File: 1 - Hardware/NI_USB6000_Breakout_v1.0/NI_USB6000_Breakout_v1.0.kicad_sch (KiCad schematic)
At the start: 19 parts, among them J1 NI_6000_CONN, J2 AIN_CONN, J3 PWR_CONN, J4 GND_CONN, J5 AIN_PWR_IN, Q1 Q_NMOS_Depletion_DGS

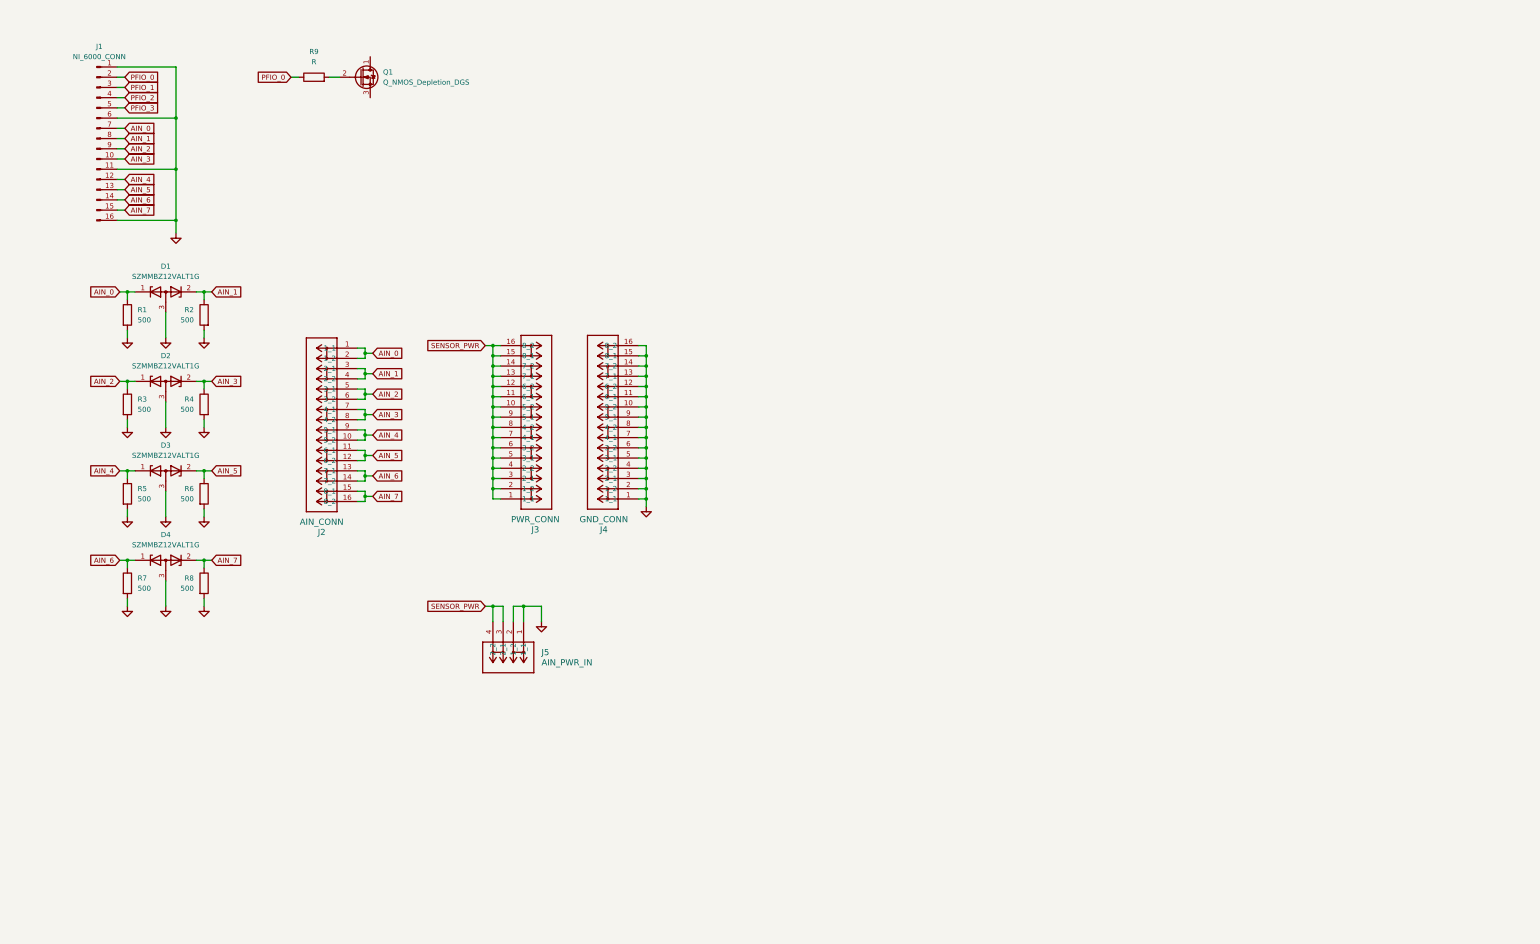
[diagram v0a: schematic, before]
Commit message: USB 6000 Breakout work
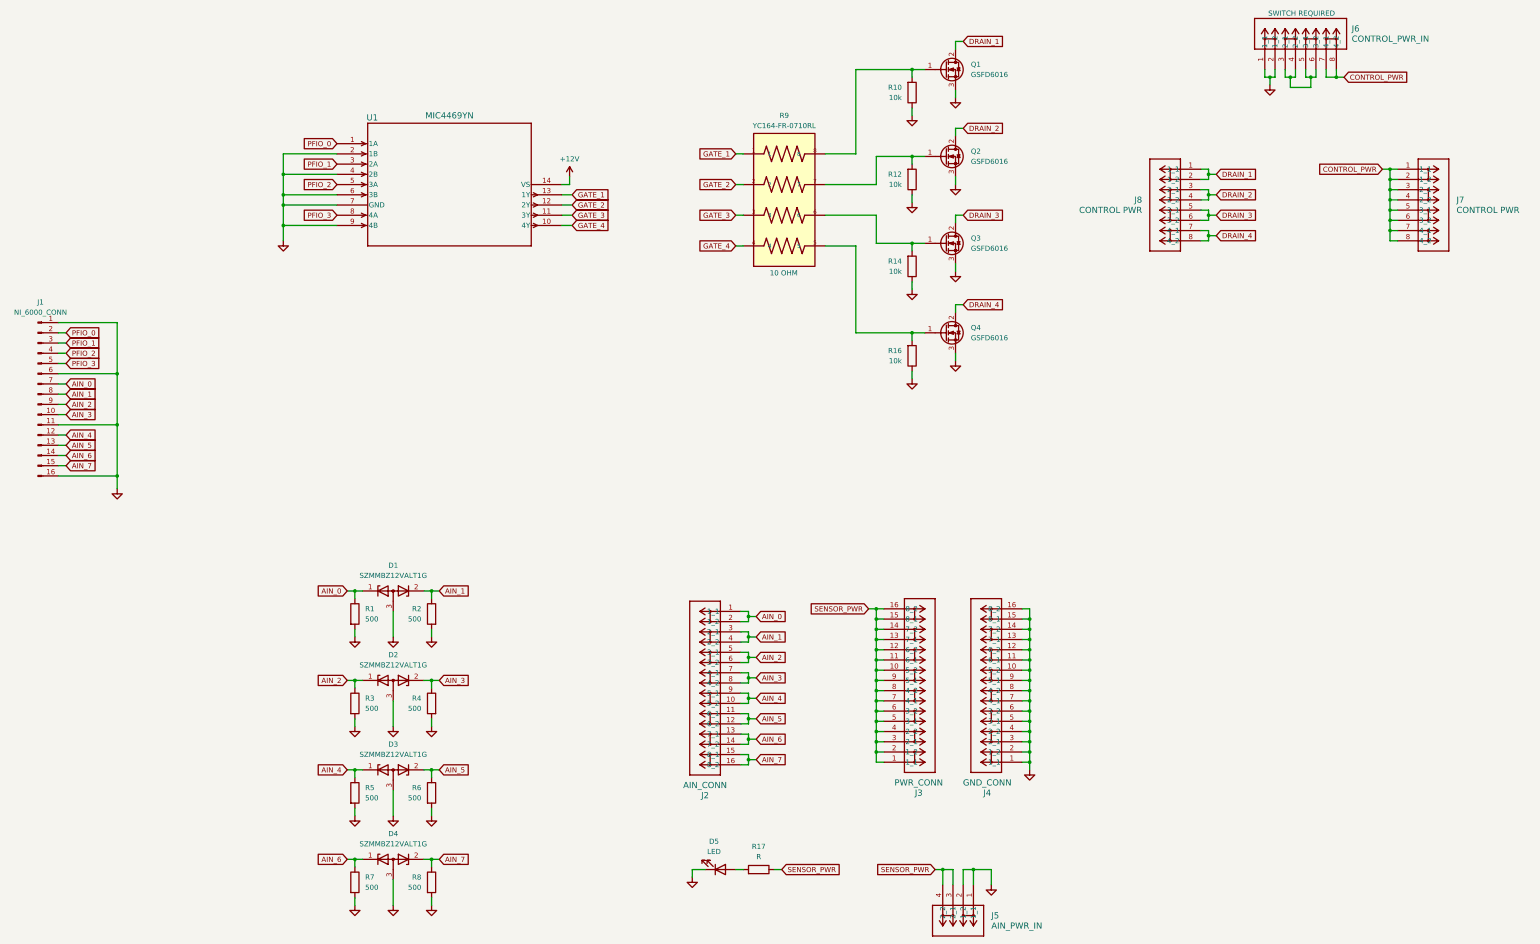
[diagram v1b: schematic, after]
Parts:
- removed Q1: Q_NMOS_Depletion_DGS, symbol Transistor_FET_Other:Q_NMOS_Depletion_DGS
- removed R9: R, symbol Device:R
- added D5: LED, symbol Device:LED
- added J6: CONTROL_PWR_IN, WAGO_2601_1104:CONN4_2601-1104_WAG, symbol WAGO_2601_1104:2601-1104
- added J7, J8: CONTROL PWR, CONN4_2601-3104_WAG, symbol 2601_3104:2601-3104
- added Q1, Q2, Q3, Q4: GSFD6016, Package_TO_SOT_SMD:TO-252-2, symbol Transistor_FET:Q_NMOS_GDS
- added R10, R12, R14, R16: 10k, symbol Device:R
- added R17: R, symbol Device:R
- added R9: YC164-FR-0710RL, YC164_FR_0710RZ:RESCAXE80P320X160X70-8N, symbol YC164_FR_0710RZ:YC164-FR-0710RL
- added U1: MIC4469YN, MIC4469YN:PDIP-14_MCL, symbol MIC4469YN:MIC4469YN
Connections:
- net GND: now also D5.1 (K), J6.1 (1_1), J6.2 (1_2), Q1.3 (S), Q2.3 (S), Q3.3 (S), Q4.3 (S), R10.1, R12.1, R14.1, R16.1, U1.2 (1B), U1.4 (2B), U1.6 (3B), U1.7 (GND), U1.9 (4B)
- net PFIO_0: now also U1.1 (1A)
- net PFIO_1: now also U1.3 (2A)
- net PFIO_2: now also U1.5 (3A)
- net PFIO_3: now also U1.8 (4A)
- net SENSOR_PWR: now also R17.1
- new net: Q4.1 (G), R16.2, R9.5
- new net: Q3.1 (G), R14.2, R9.6
- new net: Q2.1 (G), R12.2, R9.7
- new net: Q1.1 (G), R10.2, R9.8
- new net: D5.2 (A), R17.2
- new net: J6.3 (2_1), J6.4 (2_2), J6.5 (3_1), J6.6 (3_2)
- new net +12V: U1.14 (VS)
- new net CONTROL_PWR: J6.7 (4_1), J6.8 (4_2), J7.1 (1_1), J7.2 (1_2), J7.3 (2_1), J7.4 (2_2), J7.5 (3_1), J7.6 (3_2), J7.7 (4_1), J7.8 (4_2)
- new net DRAIN_1: J8.1 (1_1), J8.2 (1_2), Q1.2 (D)
- new net DRAIN_2: J8.3 (2_1), J8.4 (2_2), Q2.2 (D)
- new net DRAIN_3: J8.5 (3_1), J8.6 (3_2), Q3.2 (D)
- new net DRAIN_4: J8.7 (4_1), J8.8 (4_2), Q4.2 (D)
- new net GATE_1: R9.1, U1.13 (1Y)
- new net GATE_2: R9.2, U1.12 (2Y)
- new net GATE_3: R9.3, U1.11 (3Y)
- new net GATE_4: R9.4, U1.10 (4Y)
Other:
- note added: "10 OHM"
- note added: "SWITCH REQUIRED"
- moved on the sheet: D1, D2, D3, D4, J1, J2, J3, J4, J5, R1, R2, R3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

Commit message: USB 6000 KiCAD Work
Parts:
- removed D5: LED, symbol Device:LED
- added D10, D6, D7, D9: D, symbol Device:D
- added D11, D12, D5, D8: D_Zener, symbol Device:D_Zener
- added D13, D14: LED, symbol Device:LED
- added R15: R, symbol Device:R
- added TP1, TP10, TP11, TP12, TP13, TP14, TP15, TP16, TP17, TP18, TP19, TP2, TP20, TP21, TP22, TP23, TP3, TP4, TP5, TP6, TP7, TP8, TP9: TestPoint, symbol Connector:TestPoint
- renumbered R12 to R11, R14 to R12, R16 to R13, R17 to R14
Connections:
- net AIN_0: now also TP4.1
- net AIN_1: now also TP5.1
- net AIN_2: now also TP6.1
- net AIN_3: now also TP7.1
- net AIN_4: now also TP8.1
- net AIN_5: now also TP9.1
- net AIN_6: now also TP10.1
- net AIN_7: now also TP11.1
- net CONTROL_PWR: now also D11.2 (A), D12.2 (A), D5.2 (A), D8.2 (A), R15.1, TP3.1
- net DRAIN_1: now also D6.2 (A), TP20.1
- net DRAIN_2: now also D7.2 (A), TP21.1
- net DRAIN_3: now also D9.2 (A), TP22.1
- net DRAIN_4: now also D10.2 (A), TP23.1
- net GATE_1: now also TP16.1
- net GATE_2: now also TP17.1
- net GATE_3: now also TP18.1
- net GATE_4: now also TP19.1
- net GND: now also D13.1 (K), D14.1 (K), TP1.1
- net PFIO_0: now also TP12.1
- net PFIO_1: now also TP13.1
- net PFIO_2: now also TP14.1
- net PFIO_3: now also TP15.1
- net SENSOR_PWR: now also TP2.1
- net at R14.2: now also D13.2 (A)
- new net: D10.1 (K), D12.1 (K)
- new net: D11.1 (K), D9.1 (K)
- new net: D14.2 (A), R15.2
- new net: D7.1 (K), D8.1 (K)
- new net: D5.1 (K), D6.1 (K)
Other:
- note added: "AIN CONNS"
- note added: "CLAMPING DIODE CIRCUITRY"
- note added: "CONTROL CONNS"
- note added: "CURRENT IN CIRCUITRY"
- note added: "Horz."
- note added: "INDICATION LEDS"
- note added: "MOSFET DRIVER"
- note added: "TEST POINTS"
- note added: "USB 6000 CONN"
- note added: "Vert."
- moved on the sheet: D1, D2, D3, D4, J1, J2, J3, J4, J5, J6, J7, J8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
